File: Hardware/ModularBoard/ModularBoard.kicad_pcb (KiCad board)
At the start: 2 copper layers, 20.3 x 58.4 mm, 16 parts, among them IC1 WS2811-5050, IC2 WS2811-5050, IC3 WS2811-5050, IC4 WS2811-5050, IC5 ATTINY85-P, J1 GSG-USB-MICRO-B, K1 CONN_3, K2 CONN_3, K3 CONN_3, K4 CONN_3, P1 CONN_3X2, X1 CRYSTAL

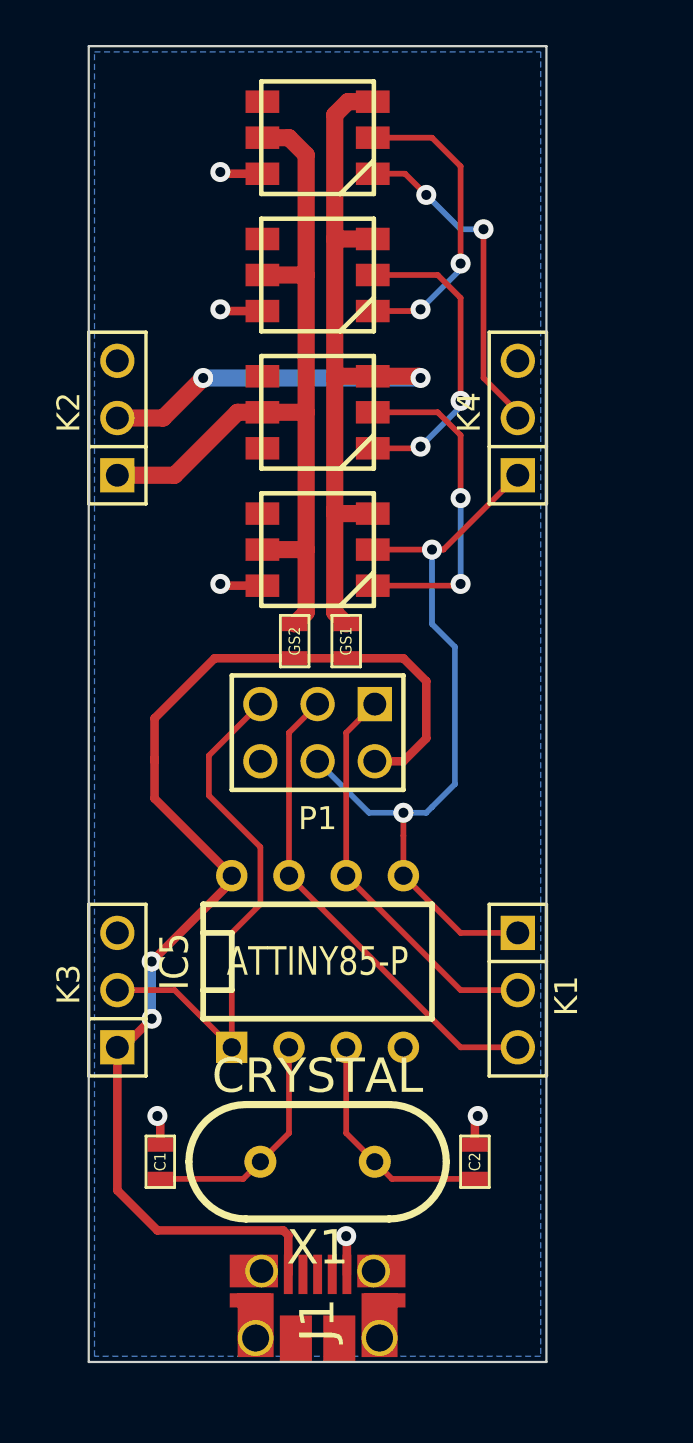
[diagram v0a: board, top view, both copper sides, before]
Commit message: Its compact! Fits in 5x5cm square
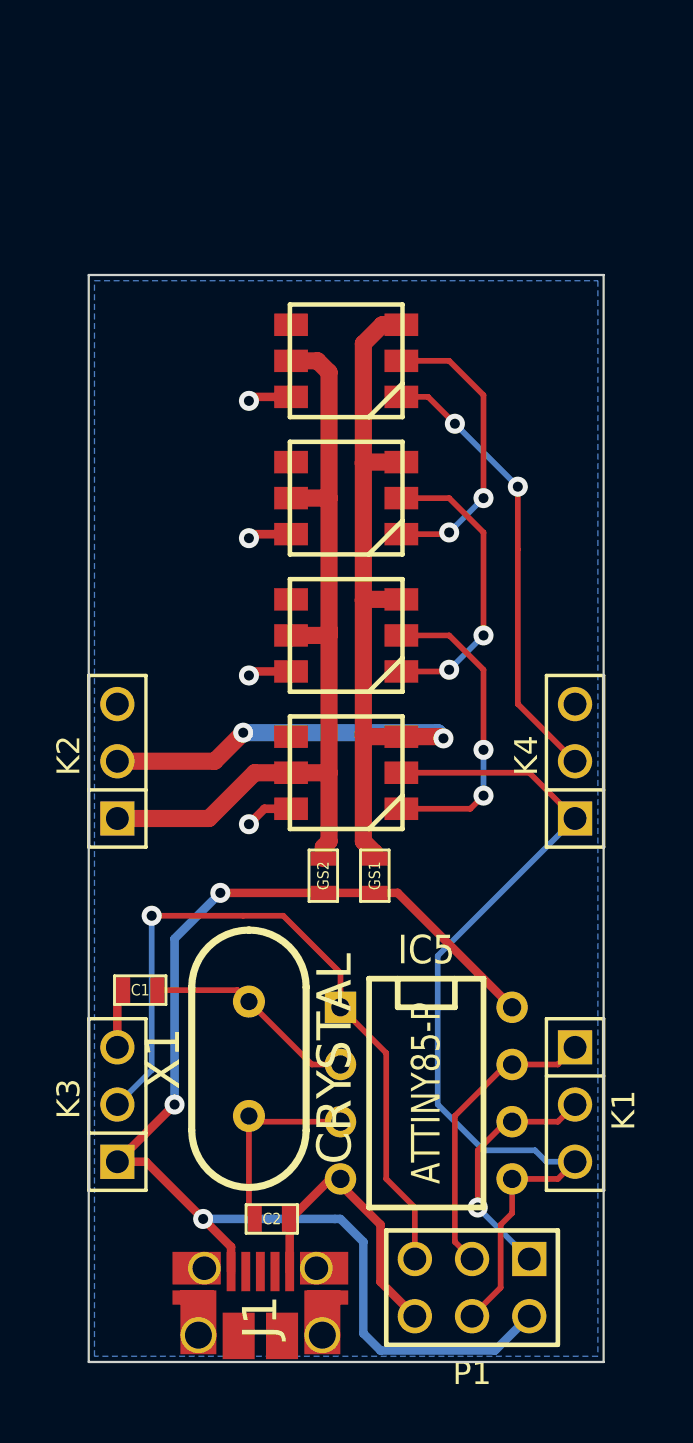
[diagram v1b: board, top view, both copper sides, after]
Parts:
- moved P1 25.6 mm to (232.9, 164.3)
- moved K4 15.5 mm to (237.5, 141.0)
- moved K2 15.2 mm to (217.2, 141.0)
- moved GS1 10.5 mm to (228.6, 146.1)
- moved GS2 10.5 mm to (226.3, 146.1)
- moved IC1 9.99 mm to (227.3, 141.5)
- moved IC2 9.99 mm to (227.3, 135.4)
- moved IC3 9.99 mm to (227.3, 129.3)
- moved IC4 9.99 mm to (227.3, 123.2)
- moved C2 9.37 mm to (224.0, 161.3), turned to 0 degrees
- moved C1 7.67 mm to (218.2, 151.1), turned to 180 degrees
- moved IC5 7.58 mm to (230.9, 155.7), turned to 270 degrees
- moved K1 5.68 mm to (237.5, 156.2)
- moved X1 5.49 mm to (223.0, 154.2), turned to 90 degrees
- moved K3 5.08 mm to (217.2, 156.2)
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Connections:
- K1 pad 1: /MOSI -> /SCK
- K1 pad 3: /SCK -> /MOSI
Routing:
- net GND: track 10.1 -> 23.4 mm, vias 6 -> 4
- net /RESET: track 23.8 -> 32.5 mm, vias 0 -> 1
- net /SCK: track 21.5 -> 13.3 mm
- net /MISO: track 17.9 -> 10.9 mm, vias 0 -> 1
- net /MOSI: track 35.1 -> 40.9 mm, vias 2 -> 0
- net /DO: track 14.9 -> 20.1 mm
- net +5V: track 53.5 -> 56.5 mm, vias 2 -> 3
- net N-0000018: track 10.4 -> 8.85 mm
- net N-000005: track 14.9 -> 13.8 mm
- net VCC: track 46.4 -> 47.5 mm
- net N-0000017: track 10.4 -> 9.50 mm
- net VDD: track 36.7 -> 37.5 mm
- net N-0000011: track 13.8 -> 13.2 mm
- net N-0000012: track 13.7 -> 13.2 mm
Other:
- board size 20.3 x 58.4 mm -> 22.9 x 48.3 mm
